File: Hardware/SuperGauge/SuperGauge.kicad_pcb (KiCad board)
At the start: 2 copper layers, 51 x 51 mm, 31 parts, among them J101 USBC, J102 MainConn, J103 Tag Connect, U102 NCV1117ST50T3G, U103 ATmega16U2, U104 TB6612FNG, Y101 Crystal_GND24

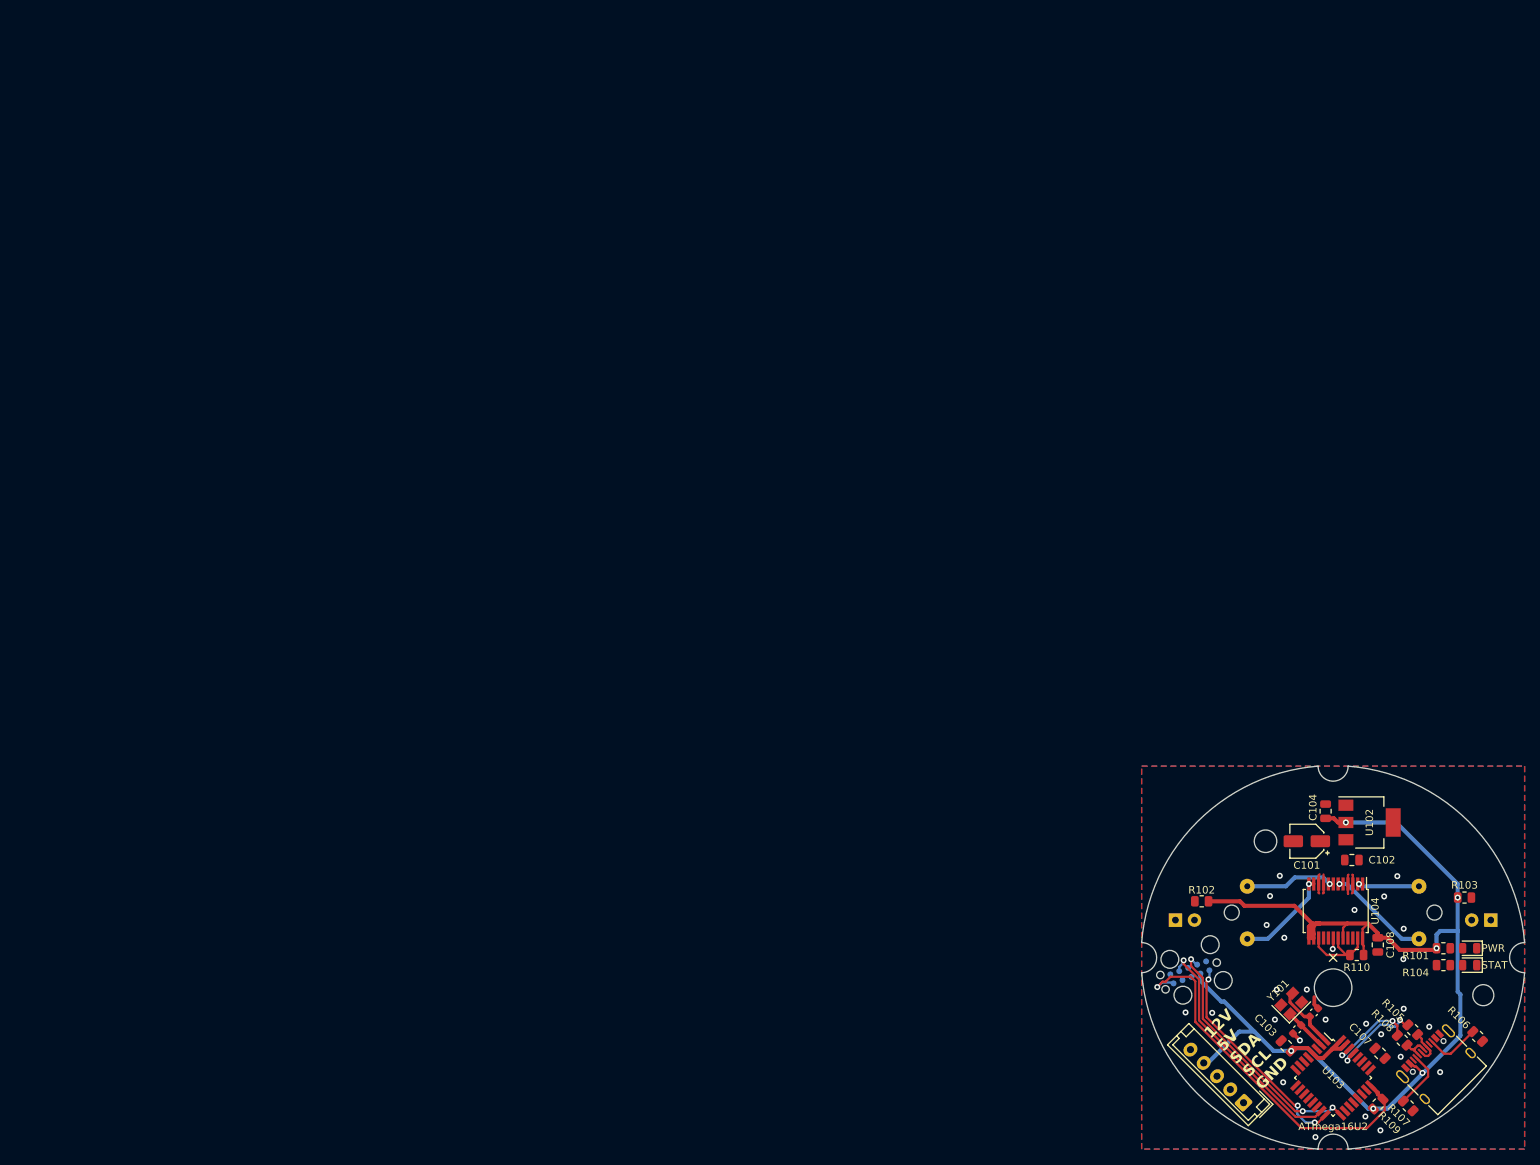
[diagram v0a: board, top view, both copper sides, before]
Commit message: Connect all
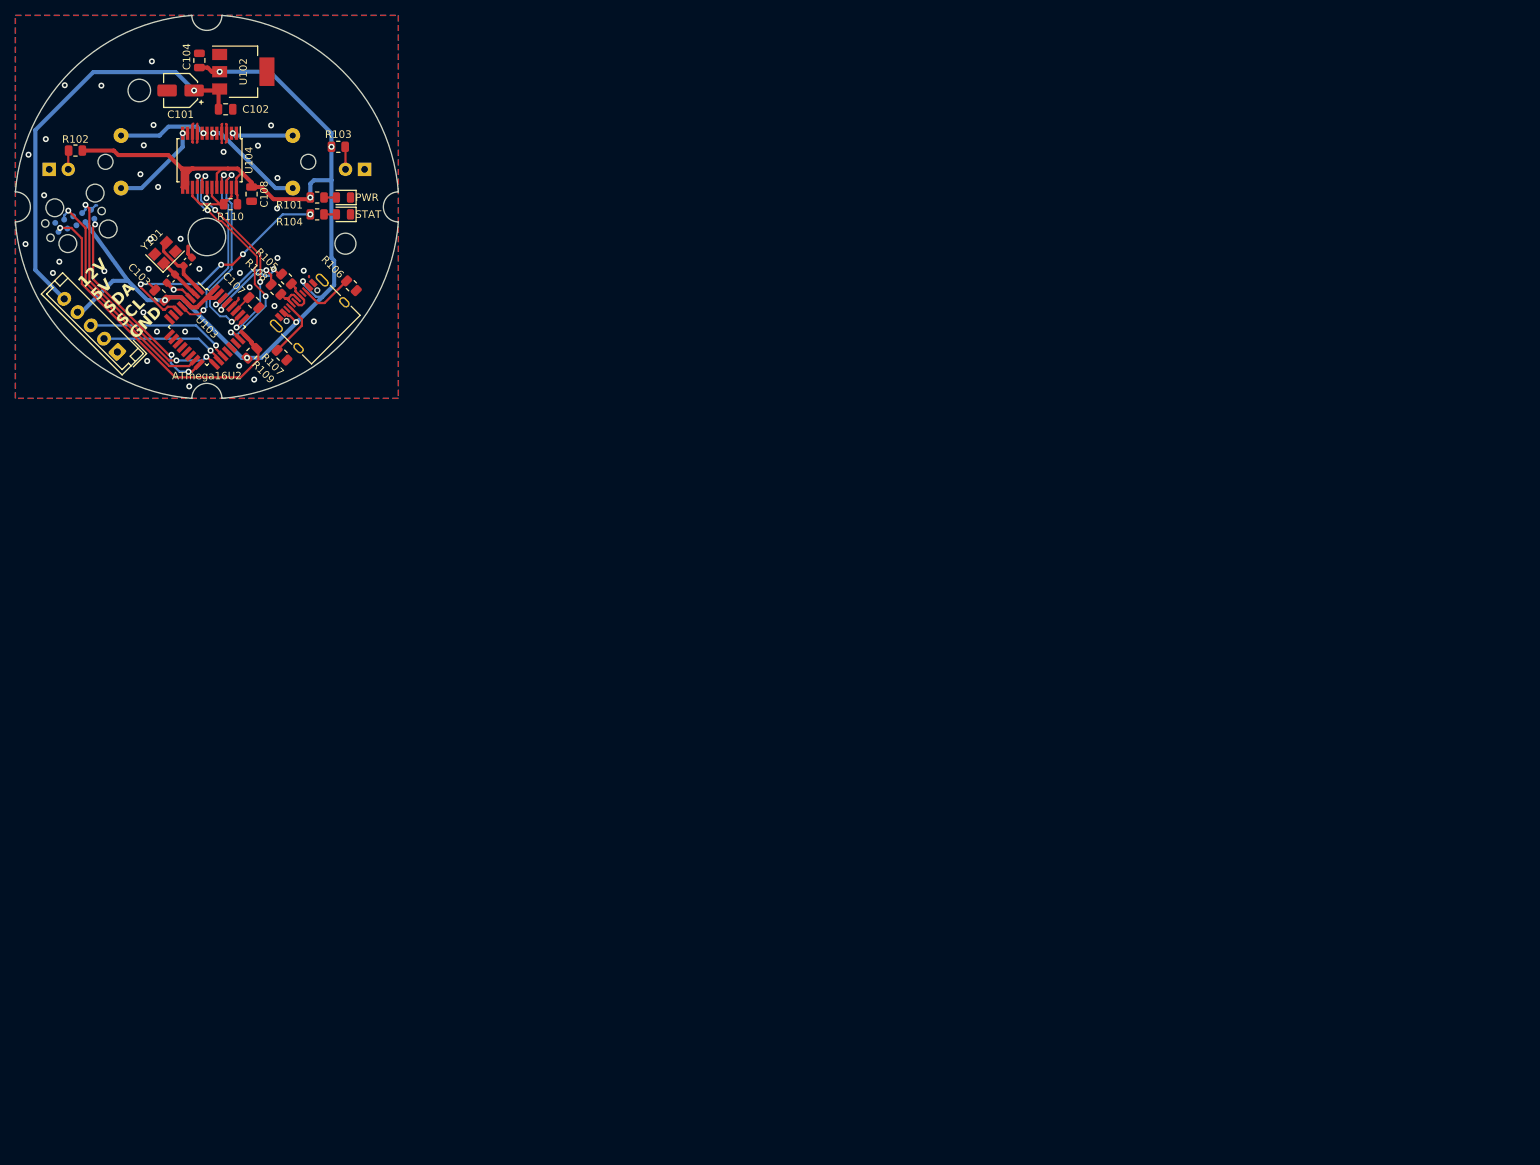
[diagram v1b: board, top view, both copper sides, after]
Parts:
- moved C101 180.2 mm to (-3.48, -15.5)
- moved C102 180.2 mm to (2.52, -13.0)
- moved C103 180.2 mm to (-6.23, 11.8)
- moved C104 180.2 mm to (-0.98, -19.5)
- moved C107 180.2 mm to (6.27, 12.8)
- moved D101 180.2 mm to (18.2, -1.23)
- moved D102 180.2 mm to (-21.0, -4.97)
- moved D103 180.2 mm to (21.0, -4.97)
- moved D104 180.2 mm to (18.2, 1.02)
- moved G*** 180.2 mm to (-3.98, 18.0)
- moved J101 180.2 mm to (14.5, 15.0)
- moved R101 180.2 mm to (14.7, -1.23)
- moved R102 180.2 mm to (-17.5, -7.47)
- moved R103 180.2 mm to (17.5, -7.97)
- moved R104 180.2 mm to (14.7, 1.02)
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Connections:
- U103 pad 18: unconnected-(U103-PB4-Pad18) -> /SCL
- U103 pad 19: unconnected-(U103-PB5-Pad19) -> /SDA
- U103 pad 23: unconnected-(U103-PC6-Pad23) -> /BIN2
- U103 pad 25: unconnected-(U103-PC5-Pad25) -> /BIN1
- U103 pad 26: unconnected-(U103-PC4-Pad26) -> /AIN2
- U103 pad 5: unconnected-(U103-PC2-Pad5) -> /AIN1
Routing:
- net +12V: track 0.00 -> 55.7 mm, vias 0 -> 1
- net Net-(U103-PD0): track 0.00 -> 33.4 mm, vias 0 -> 4
- net /BIN2: track 0.00 -> 31.1 mm, vias 0 -> 4
- net /BIN1: track 0.00 -> 28.8 mm, vias 0 -> 4
- net /AIN2: track 0.00 -> 26.4 mm, vias 0 -> 2
- net /AIN1: track 0.00 -> 25.0 mm, vias 0 -> 2
- net /SDA: track 0.00 -> 19.6 mm, vias 0 -> 1
- net /SCL: track 0.00 -> 16.6 mm, vias 0 -> 1
- net GND: track 15.1 -> 21.7 mm, vias 27 -> 38
- net +5V: track 161.0 -> 167.4 mm, vias 6 -> 7
- net /ICSP_RST: track 49.9 -> 43.8 mm
- net Net-(D103-A): track 0.00 -> 3.02 mm
- net Net-(D102-A): track 0.00 -> 2.52 mm
- net Net-(U103-UCAP): track 0.00 -> 2.48 mm
- net Net-(D104-A): track 0.00 -> 1.65 mm
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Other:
- outline, holes or cut-outs redrawn
